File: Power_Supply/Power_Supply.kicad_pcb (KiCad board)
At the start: 2 copper layers, 50 x 100 mm, 39 parts, among them J1 Cable_PAD, J2 Cable_PAD, J3 Cable_PAD, J4 CONN_01X03, J5 jack, J6 Cable_PAD, J7 Cable_PAD, J8 Cable_PAD, Q1 TIP41C, Q2 BD139, Q3 BC548, Q4 BC558, Q5 BC558, SW1 SW_SPST, SW2 SW_Push, U1 LM358

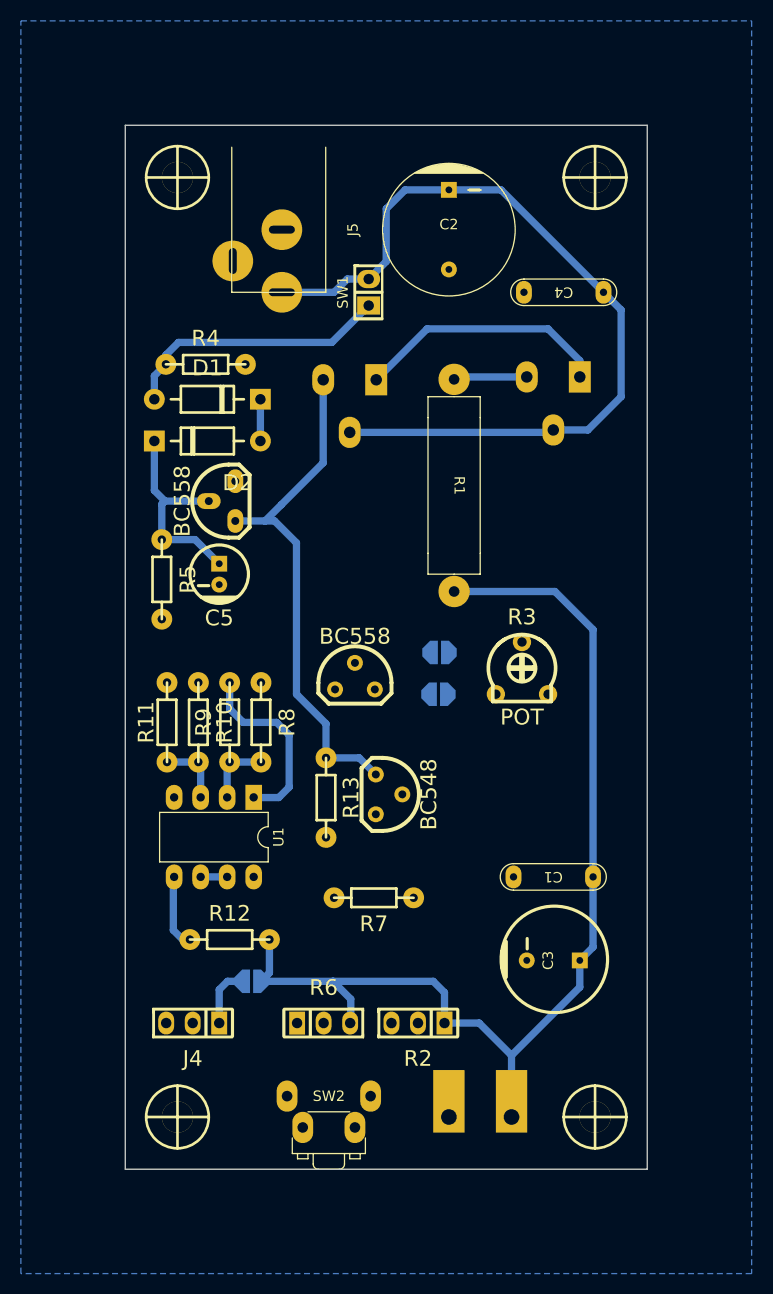
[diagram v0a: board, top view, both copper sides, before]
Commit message: new
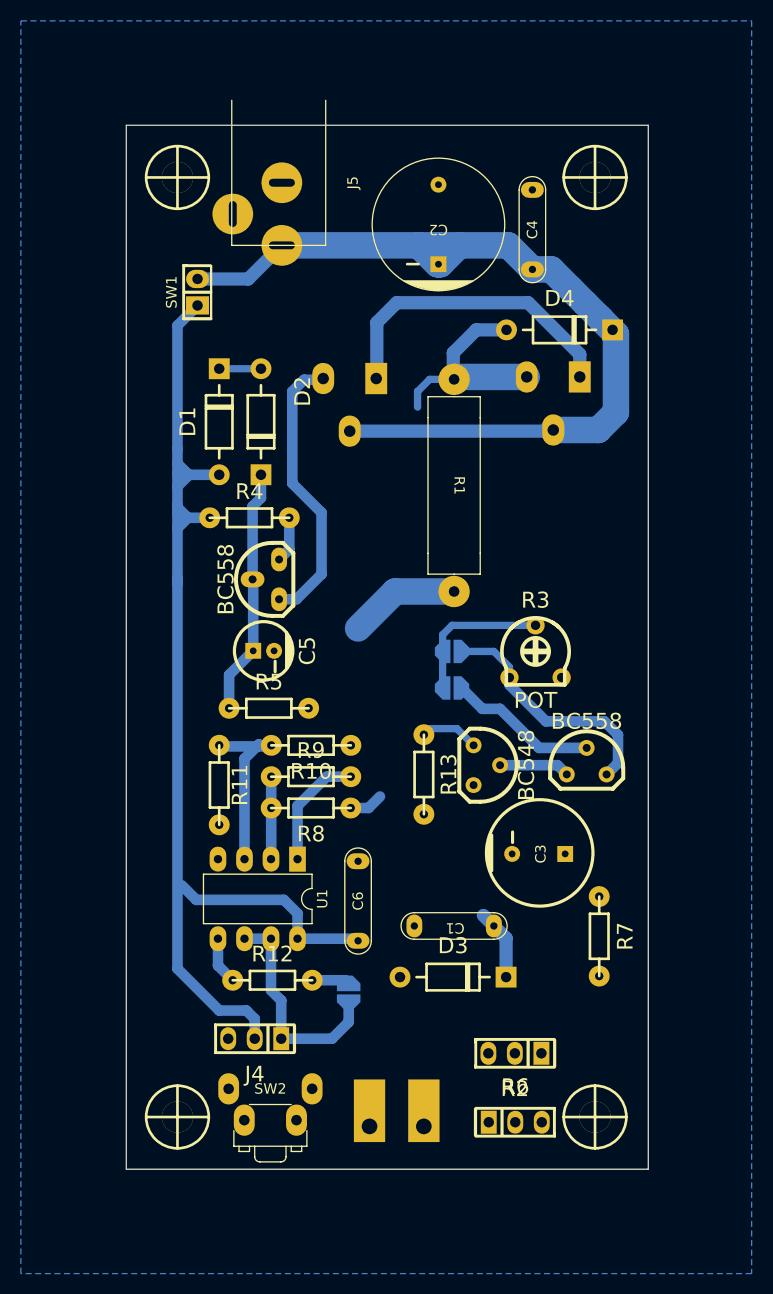
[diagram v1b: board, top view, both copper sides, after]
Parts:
- added C6: 100n, Modified_Footprints:C_POL, F.Cu at (172.3, 114.3)
- added D3: RECTIFIER_DIODE, EESTN5:DO-41, F.Cu at (181.4, 121.6)
- added D4: RECTIFIER_DIODE, EESTN5:DO-41, F.Cu at (191.6, 59.6)
- moved Q5 23.6 mm to (194.2, 101.5)
- moved R7 21.9 mm to (195.4, 117.7), turned to -90 degrees
- moved R6 20.7 mm to (187.4, 135.5)
- moved SW1 16.4 mm to (156.6, 56.0)
- moved R5 16.0 mm to (163.8, 95.8), turned to 0 degrees
- moved R4 15.3 mm to (161.9, 77.6)
- moved R10 11.0 mm to (167.8, 99.4), turned to 180 degrees
- moved C1 10.6 mm to (181.5, 116.7)
- moved C3 10.3 mm to (189.6, 109.8)
- moved Q3 9.77 mm to (184.0, 101.3)
- moved R2 9.72 mm to (187.3, 128.9)
- moved R13 9.63 mm to (178.6, 102.2)
- moved R8 9.51 mm to (167.8, 105.4), turned to 180 degrees
- moved R9 9.37 mm to (167.8, 102.4), turned to 0 degrees
- moved JP3 9.36 mm to (171.4, 123.1), turned to 180 degrees
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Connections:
- R2 pad 1: /-R -> Net-(R2-Pad1)
- R2 pad 3: Net-(R2-Pad3) -> /-R
- R3 pad 1: Net-(R2-Pad3) -> Net-(JP1-A)
- R3 pad 3: Net-(JP1-A) -> Net-(R2-Pad1)
- U1 pad 8: VCC -> /SW_OUT
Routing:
- net /SW_OUT: track 26.1 -> 110.2 mm
- net /-R: track 102.5 -> 25.2 mm
- net Net-(JP1-A): track 24.3 -> 53.4 mm
- net Net-(Q2-B): track 49.8 -> 34.5 mm
- net Net-(JP2-B): track 0.00 -> 14.5 mm
- net Net-(JP1-B): track 0.00 -> 14.4 mm
- net /+R: track 7.06 -> 21.1 mm
- net Net-(J4-P1): track 8.27 -> 21.5 mm
- net Net-(U1A-+): track 6.47 -> 17.9 mm
- net VCC: track 80.0 -> 90.5 mm
- net Net-(Q3-B): track 0.00 -> 6.76 mm
- net Net-(R9-Pad2): track 18.1 -> 11.4 mm
- net Net-(Q4-E): track 0.00 -> 4.40 mm
- net Net-(D2-K): track 20.6 -> 23.7 mm
- net /V+: track 7.10 -> 4.56 mm
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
